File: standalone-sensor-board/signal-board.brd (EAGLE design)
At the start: 26 x 93.5 mm, 25 parts, among them J1 sensors, J3 to_next_board, J4 to_controller, U1 CD4051BE

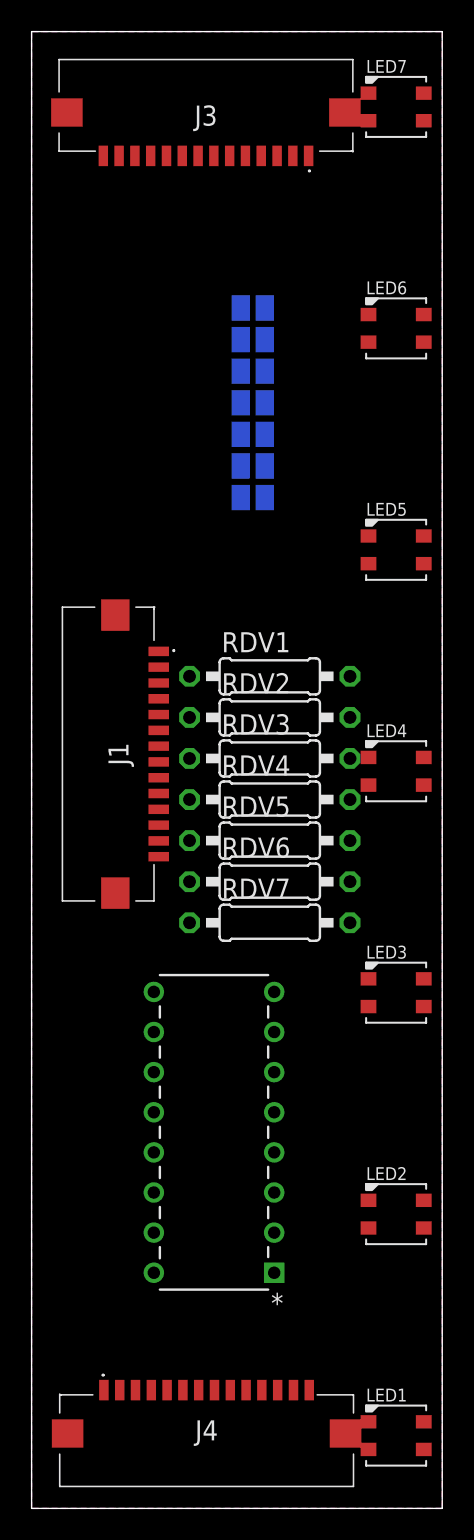
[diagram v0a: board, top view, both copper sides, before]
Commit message: signal board routing
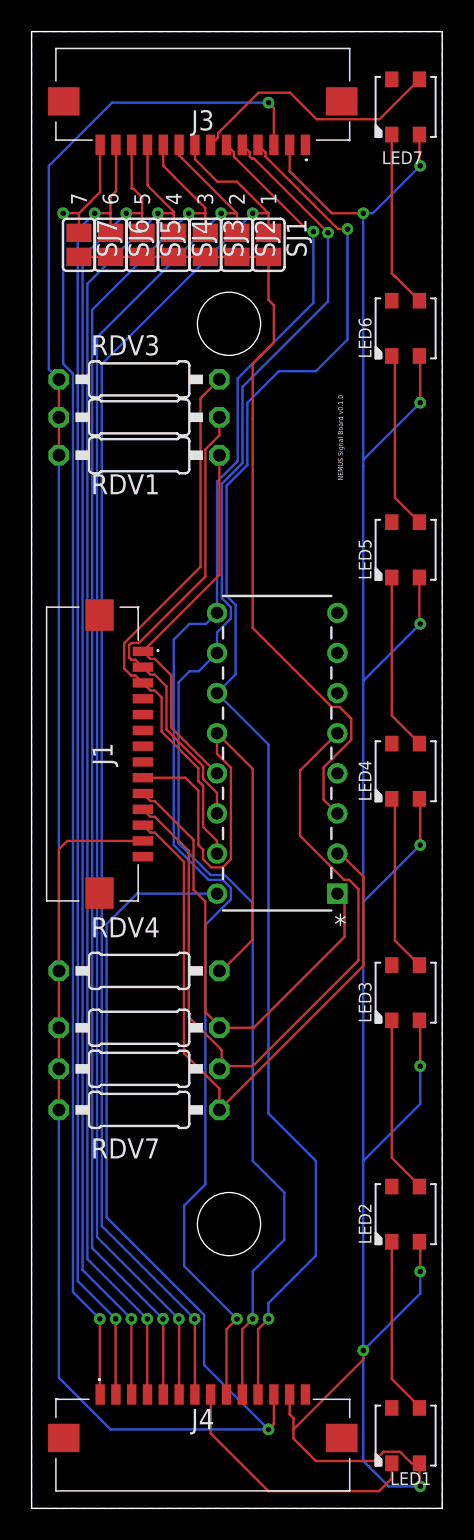
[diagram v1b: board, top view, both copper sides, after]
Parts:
- moved RDV3 25.4 mm to (6.81, 71.5)
- moved U1 24.3 mm to (19.4, 38.9)
- moved RDV2 20.7 mm to (6.81, 69.1)
- moved SJ7 19.4 mm to (3.00, 80.0), flipped to the top, turned to 270 degrees
- moved SJ6 16.6 mm to (5.00, 80.0), flipped to the top, turned to 270 degrees
- moved RDV1 16.3 mm to (6.81, 66.7)
- moved RDV5 14.5 mm to (6.81, 30.4)
- moved RDV6 14.5 mm to (6.81, 27.8)
- moved RDV7 14.5 mm to (6.81, 25.2)
- moved SJ5 13.9 mm to (7.00, 80.0), flipped to the top, turned to 270 degrees
- moved RDV4 13.6 mm to (6.81, 34.0)
- moved SJ4 11.2 mm to (9.00, 80.0), flipped to the top, turned to 270 degrees
- moved SJ3 8.54 mm to (11.0, 80.0), flipped to the top, turned to 270 degrees
- moved SJ2 6.08 mm to (13.0, 80.0), flipped to the top, turned to 270 degrees
- moved SJ1 4.12 mm to (15.0, 80.0), flipped to the top, turned to 270 degrees
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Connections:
- net 3V: now also J3.2; no longer J3.13
- net A: now also J3.4; no longer J3.11
- net B: now also J3.5; no longer J3.10
- net C: now also J3.6; no longer J3.9
- net DOUT: now also J3.7; no longer J3.8
- net GND: now also J3.1; no longer J3.14
- net S1: now also J3.8; no longer J3.7
- net S2: now also J3.9; no longer J3.6
- net S3: now also J3.10; no longer J3.5
- net S4: now also J3.11; no longer J3.4
- net S5: now also J3.12; no longer J3.3
- net S6: now also J3.13; no longer J3.2
- net S7: now also J3.14; no longer J3.1
- net VCC: now also J3.3; no longer J3.12
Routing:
- net VCC: track 0.00 -> 169.6 mm, vias 0 -> 2
- net 3V: track 0.00 -> 160.9 mm, vias 0 -> 9
- net A: track 0.00 -> 91.2 mm, vias 0 -> 2
- net C: track 0.00 -> 90.7 mm, vias 0 -> 2
- net B: track 0.00 -> 90.6 mm, vias 0 -> 2
- net S1: track 0.00 -> 90.4 mm, vias 0 -> 2
- net S2: track 0.00 -> 88.3 mm, vias 0 -> 2
- net S3: track 0.00 -> 86.9 mm, vias 0 -> 2
- net S4: track 0.00 -> 85.5 mm, vias 0 -> 2
- net S5: track 0.00 -> 84.1 mm, vias 0 -> 2
- net S6: track 0.00 -> 83.0 mm, vias 0 -> 2
- net S7: track 0.00 -> 82.9 mm, vias 0 -> 2
- net SIG: track 0.00 -> 51.9 mm
- net C5: track 0.00 -> 47.2 mm
- net C6: track 0.00 -> 41.0 mm
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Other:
- board text added: "NEMUS Signal Board v0.1.0"
- board text removed: "NEMUS Face Board v0.1.1"
